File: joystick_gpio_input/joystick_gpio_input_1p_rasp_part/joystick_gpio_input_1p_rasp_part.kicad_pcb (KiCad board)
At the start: 2 copper layers, 11.7 x 23.2 mm, 3 parts, among them J10 Conn_01x14, J6 Conn_02x09_Odd_Even, J8 Conn_01x14

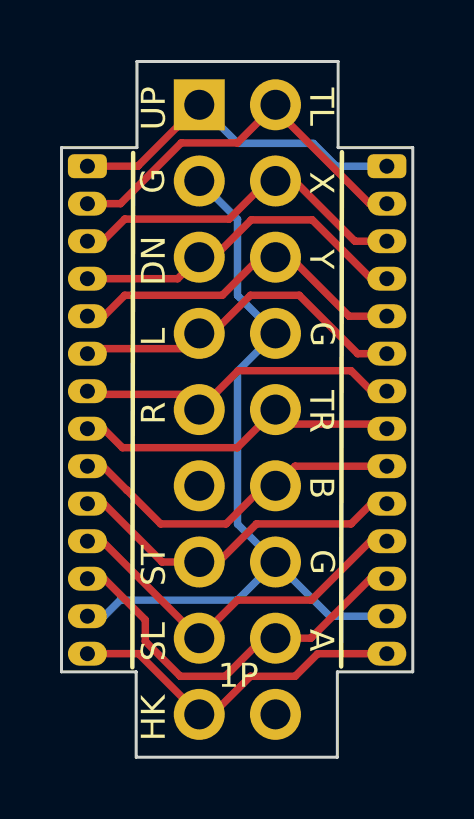
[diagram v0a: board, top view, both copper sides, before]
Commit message: gpio 입력 보드 미세 조정
Signed-off-by: Ju, Gyeong-min <jcmh74@gmail.com>
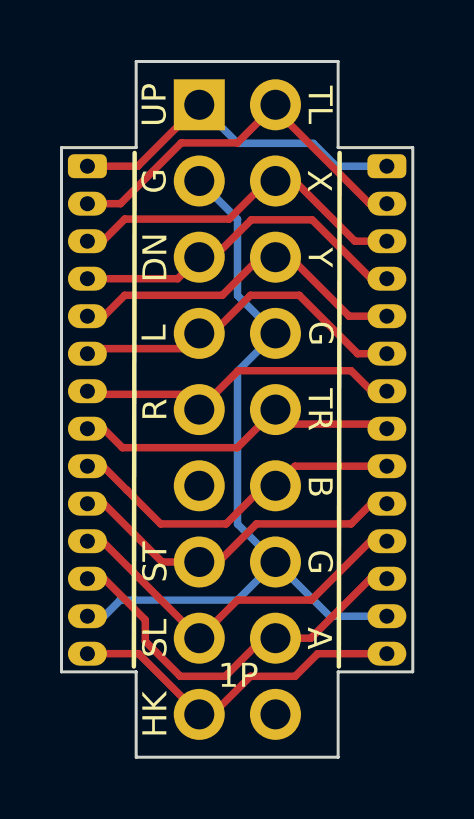
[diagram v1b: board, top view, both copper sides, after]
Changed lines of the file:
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@@
     )
   )
-  (gr_line (start 152.2222 90.551) (end 152.1968 107.696)
+  (gr_line (start 152.146 90.5764) (end 152.1206 107.696)
     (stroke (width 0.15) (type default)) (layer "F.SilkS"))
-  (gr_line (start 145.2626 90.5764) (end 145.2372 107.7214)
+  (gr_line (start 145.3134 90.5764) (end 145.288 107.696)
     (stroke (width 0.15) (type default)) (layer "F.SilkS"))
   (gr_poly
     (pts
       (xy 152.0952 87.5284)
-      (xy 145.3896 87.5284)
-      (xy 145.3896 90.3986)
+      (xy 145.3642 87.5284)
+      (xy 145.3642 90.3986)
       (xy 142.875 90.3986)
       (xy 142.875 107.8738)
       (xy 145.3642 107.8738)
       (xy 145.3642 110.7186)
-      (xy 152.0698 110.7186)
-      (xy 152.0698 107.8738)
+      (xy 152.0952 110.7186)
+      (xy 152.0952 107.8738)
       (xy 154.5844 107.8738)
       (xy 154.5844 90.3986)
@@
     )
     (stroke (width 0.1) (type solid)) (fill none) (layer "Edge.Cuts"))
-  (gr_text "G" (at 151.5618 96.6166 -90) (layer "F.SilkS")
+  (gr_text "G" (at 151.511 96.5962 -90) (layer "F.SilkS")
     (effects (font (size 0.8 0.8) (thickness 0.15)))
   )
-  (gr_text "SL" (at 145.9484 106.8682 90) (layer "F.SilkS")
+  (gr_text "SL" (at 145.9992 106.7562 90) (layer "F.SilkS")
     (effects (font (size 0.8 0.8) (thickness 0.15)))
   )
@@
     (effects (font (size 0.8 0.8) (thickness 0.15)))
   )
-  (gr_text "TL" (at 151.5364 89.0374 270) (layer "F.SilkS")
+  (gr_text "TL" (at 151.4856 88.9762 270) (layer "F.SilkS")
     (effects (font (size 0.8 0.8) (thickness 0.15)))
   )
-  (gr_text "G" (at 145.923 91.5112 90) (layer "F.SilkS")
+  (gr_text "G" (at 145.9738 91.5112 90) (layer "F.SilkS")
     (effects (font (size 0.8 0.8) (thickness 0.15)))
   )
-  (gr_text "Y" (at 151.5364 94.1174 270) (layer "F.SilkS")
+  (gr_text "Y" (at 151.4856 94.0562 270) (layer "F.SilkS")
     (effects (font (size 0.8 0.8) (thickness 0.15)))
   )
-  (gr_text "UP" (at 145.9484 89.0882 90) (layer "F.SilkS")
+  (gr_text "UP" (at 145.9738 88.9762 90) (layer "F.SilkS")
     (effects (font (size 0.8 0.8) (thickness 0.15)))
   )
-  (gr_text "TR" (at 151.5364 99.1974 270) (layer "F.SilkS")
+  (gr_text "TR" (at 151.4856 99.1362 270) (layer "F.SilkS")
     (effects (font (size 0.8 0.8) (thickness 0.15)))
   )
-  (gr_text "HK" (at 145.9484 109.4082 90) (layer "F.SilkS")
+  (gr_text "HK" (at 145.9992 109.2962 90) (layer "F.SilkS")
     (effects (font (size 0.8 0.8) (thickness 0.15)))
   )
-  (gr_text "DN" (at 145.9484 94.1682 90) (layer "F.SilkS")
+  (gr_text "DN" (at 145.9992 94.0562 90) (layer "F.SilkS")
     (effects (font (size 0.8 0.8) (thickness 0.15)))
   )
-  (gr_text "A" (at 151.5364 106.8174 270) (layer "F.SilkS")
+  (gr_text "A" (at 151.4602 106.7562 270) (layer "F.SilkS")
     (effects (font (size 0.8 0.8) (thickness 0.15)))
   )
-  (gr_text "X" (at 151.5364 91.5774 270) (layer "F.SilkS")
+  (gr_text "X" (at 151.4602 91.5162 270) (layer "F.SilkS")
     (effects (font (size 0.8 0.8) (thickness 0.15)))
   )
-  (gr_text "R" (at 145.9484 99.2482 90) (layer "F.SilkS")
+  (gr_text "R" (at 145.9992 99.1362 90) (layer "F.SilkS")
     (effects (font (size 0.8 0.8) (thickness 0.15)))
   )
-  (gr_text "G" (at 151.5618 104.2112 -90) (layer "F.SilkS")
+  (gr_text "G" (at 151.4856 104.2112 -90) (layer "F.SilkS")
     (effects (font (size 0.8 0.8) (thickness 0.15)))
   )
-  (gr_text "L" (at 145.9484 96.7082 90) (layer "F.SilkS")
+  (gr_text "L" (at 145.9738 96.5962 90) (layer "F.SilkS")
     (effects (font (size 0.8 0.8) (thickness 0.15)))
   )
-  (gr_text "B" (at 151.5364 101.7374 270) (layer "F.SilkS")
+  (gr_text "B" (at 151.4856 101.7016 270) (layer "F.SilkS")
     (effects (font (size 0.8 0.8) (thickness 0.15)))
   )
-  (gr_text "ST" (at 145.9484 104.3282 90) (layer "F.SilkS")
+  (gr_text "ST" (at 145.9992 104.2162 90) (layer "F.SilkS")
     (effects (font (size 0.8 0.8) (thickness 0.15)))
   )

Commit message: joystick gpio 스크린샷 추가
Signed-off-by: Ju, Gyeong-min <jcmh74@gmail.com>
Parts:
- renumbered J6 to J1, J8 to J2, J10 to J3
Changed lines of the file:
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@@
   (paper "A4")
   (title_block
-    (title "Raspberry Pie GPIO Input Module")
+    (title "Raspberry Pie GPIO Input Module (1P Part)")
     (date "2023-03-26")
     (rev "2")
@@
   (net 13 "/1P_HK")
   (net 14 "/1P_GND")
-  (net 15 "unconnected-(J6-Pin_11-Pad11)")
-  (net 16 "unconnected-(J6-Pin_18-Pad18)")
+  (net 15 "unconnected-(J1-Pin_11-Pad11)")
+  (net 16 "unconnected-(J1-Pin_18-Pad18)")
   (footprint "joystick_gpio_input_library:conn_ex_1x14_P1.25mm_Vertical_Right_Labeled" (layer "B.Cu")
     (at 153.7208 91.0186 -90)
@@
     (property "ki_keywords" "connector")
     (attr through_hole)
-    (fp_text reference "J8" (at 8.12 -1.905 90) (layer "B.SilkS") hide
+    (fp_text reference "J2" (at 8.12 -1.905 90) (layer "B.SilkS") hide
         (effects (font (size 1 1) (thickness 0.15)) (justify mirror))
     )
@@
     (property "ki_keywords" "connector")
     (attr through_hole)
-    (fp_text reference "J6" (at -1.27 2.77) (layer "B.SilkS") hide
+    (fp_text reference "J1" (at -1.27 2.77) (layer "B.SilkS") hide
         (effects (font (size 1 1) (thickness 0.15)) (justify mirror))
     )
@@
       (net 12 "/1P_TR") (pinfunction "Pin_10") (pintype "passive"))
     (pad "11" thru_hole oval (at 0 -12.7 180) (size 1.7 1.7) (drill 1) (layers "*.Cu" "*.Mask")
-      (net 15 "unconnected-(J6-Pin_11-Pad11)") (pinfunction "Pin_11") (pintype "passive+no_connect"))
+      (net 15 "unconnected-(J1-Pin_11-Pad11)") (pinfunction "Pin_11") (pintype "passive+no_connect"))
     (pad "12" thru_hole oval (at -2.54 -12.7 180) (size 1.7 1.7) (drill 1) (layers "*.Cu" "*.Mask")
       (net 8 "/1P_B") (pinfunction "Pin_12") (pintype "passive"))
@@
       (net 13 "/1P_HK") (pinfunction "Pin_17") (pintype "passive"))
     (pad "18" thru_hole oval (at -2.54 -20.32 180) (size 1.7 1.7) (drill 1) (layers "*.Cu" "*.Mask")
-      (net 16 "unconnected-(J6-Pin_18-Pad18)") (pinfunction "Pin_18") (pintype "passive+no_connect"))
+      (net 16 "unconnected-(J1-Pin_18-Pad18)") (pinfunction "Pin_18") (pintype "passive+no_connect"))
     (model "${KICAD6_3DMODEL_DIR}/Connector_PinSocket_2.54mm.3dshapes/PinSocket_2x09_P2.54mm_Vertical.wrl"
       (offset (xyz 0 0 0))
@@
     (property "ki_keywords" "connector")
     (attr through_hole)
-    (fp_text reference "J10" (at 8.12 1.778 90) (layer "B.SilkS") hide
-        (effects (font (size 1 1) (thickness 0.15)) (justify mirror))
-    )
+    (fp_text reference "J3" (at 8.12 1.778 90) (layer "B.SilkS") hide
+        (effects (font (size 1 1) (thickness 0.15)) (justify mirror))
+    )
